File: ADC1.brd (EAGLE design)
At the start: 100 x 100 mm, 69 parts, among them IC1 STM32F303K8T6, IC2 TC7WZ07FK, IC3 ESP32-WROVER, J1 SJ-1608, J2 SJ-1608, J3 SJ-1608, J4 SJ-1608, J5 SJ-2012, J6 SJ-1608, J7 SJ-2012, J8 SJ-1608, X1 12MHz

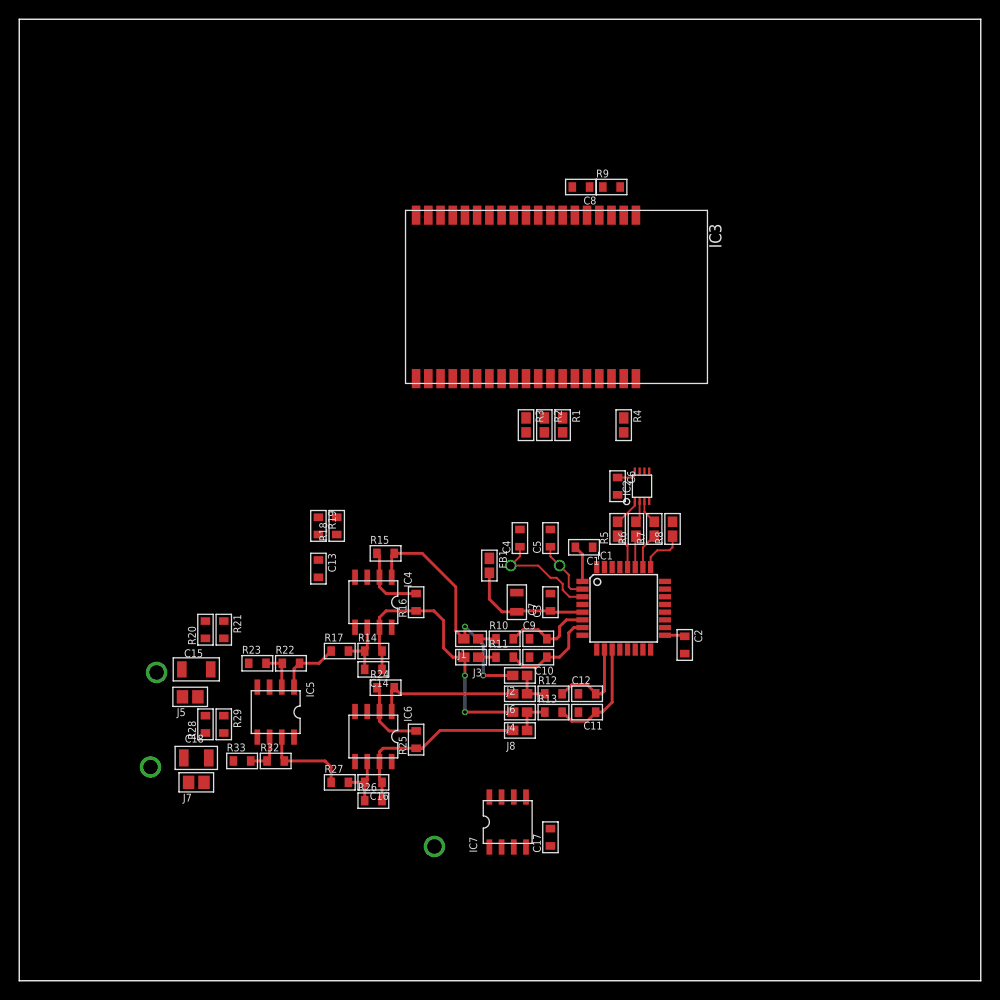
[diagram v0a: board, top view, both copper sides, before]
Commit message: ほぼ完成
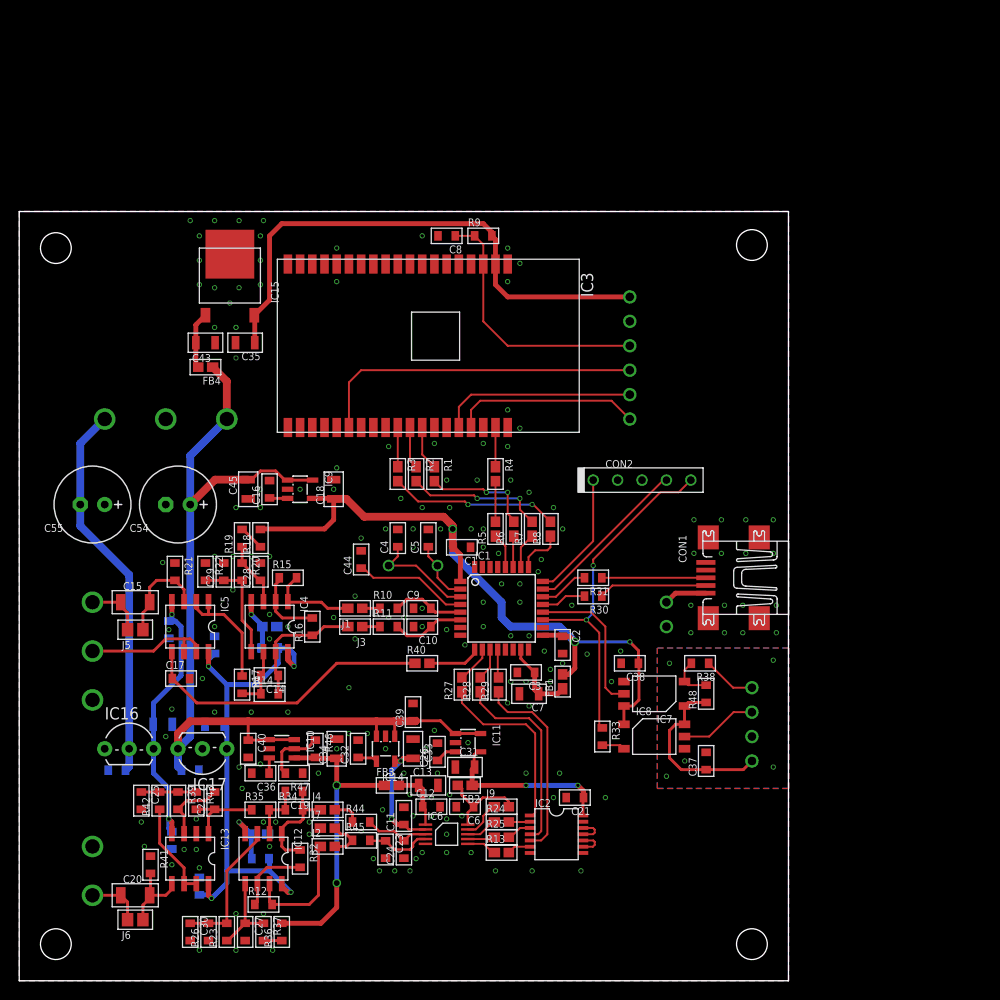
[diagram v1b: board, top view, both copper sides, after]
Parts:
- added C19, C25: 470p, my_rcl:1608
- added C20: 10u, my_rcl:3225
- added C21, C26, C27, C28, C29, C30, C32, C36, C37, C38, C39, C40, C41, C42, C44, C48, C49, C50, C51, C52, C53: 0.1u, my_rcl:1608
- added C22: 27p, my_rcl:1608
- added C23, C24: 1n, my_rcl:1608
- added C31, C33, C34, C35, C43, C45, C46, C47: 10u, my_rcl:2012
- added C54, C55: 100u, my_rcl:E2,5-8
- added CON1: USB-A, my_connector:UX60A-MB-5ST
- added CON2: SWD_CON, my_connector:SWD_CON
- added DR1, DR2, DR3, DR4: HOLE-3.2, my_connector:HOLE_3.2
- added FB2, FB3, FB4: FB, my_rcl:1608-J
- added IC10: NJM11100, my_ic:SOT23-6
- added IC11, IC9: 3.3V, my_ic:SOT23-5
- added IC12: LME49721, my_ic:SOP8
- added IC13: NJM4580, my_ic:SOP8
- added IC14: NJM12888F18, my_ic:SOT23-5
- added IC15: NJM2845-3.3, my_ic:P-HSIP3_2.30A
- added IC16: -5V, my_ic:TO-92
- added IC17: +5V, my_ic:TO-92
- added IC8: OCT_BUFFER-SO6, my_ic:SO6
- added J10, J9: SJ-1608, my_rcl:1608-J
- added R30, R31, R44, R45: 22, my_rcl:1608
- added R34, R35, R36, R37, R38, R39, R42, R43, R48: 1k, my_rcl:1608
- added R40: 0, my_rcl:1608-J
- added R41: 10k, my_rcl:1608
- added R46: 6.8k, my_rcl:1608
- added R47: 2.4k, my_rcl:1608
- added TP10: ESP_EN, my_connector:TESTPIN
- added TP11: ESP_BOOT, my_connector:TESTPIN
- added TP12: ESP_TX, my_connector:TESTPIN
- added TP13, TP20: GND, my_connector:TESTPIN
- added TP14: ESP_RX, my_connector:TESTPIN
- added TP15, TP16, TP18: GND, my_connector:TESTPIN-BIG
- added TP17: V+, my_connector:TESTPIN-BIG
- added TP19: V-, my_connector:TESTPIN-BIG
- added TP4: VBUS, my_connector:TESTPIN
- added TP5: UART_3V3, my_connector:TESTPIN
- added TP6: UART_RX, my_connector:TESTPIN
- added TP7: UART_GND, my_connector:TESTPIN
- added TP8: UART_TX, my_connector:TESTPIN
- added TP9: +3V3D, my_connector:TESTPIN
- C11: value 1n -> 0.1u
- C12: value 1n -> 3300p
- C13: value 0.1u -> 1u; device my_rcl:1608 -> my_rcl:2012
- C14: value (none) -> 27p
- C16: value (none) -> 0.1u
- C17: value (none) -> 470p
- C18: device my_rcl:3216 -> my_rcl:2012
- C7: value 1u -> 10u
- IC1: value STM32F303K8T6 -> STM32G431KB
- IC2: value TC7WZ07FK -> 7404; device my_ic:SOT765 -> my_ic:TSSOP14
- IC4: value (none) -> LME49721
- IC5: value (none) -> NJM4580
- IC6: value (none) -> MCP331X1; device my_ic:SOP8 -> my_ic:MSOP10
- IC7: value (none) -> OCT_BUFFER-SO6; device my_ic:SOP8 -> my_ic:SO6
- J5: value SJ-2012 -> IN3_DC
- J6: value SJ-1608 -> IN1_DC; device my_rcl:1608-J -> my_rcl:2012-J
- J7: value SJ-2012 -> SJ-1608; device my_rcl:2012-J -> my_rcl:1608-J
- R12: value 10 -> 1k
- R13: value 10 -> 37; device my_rcl:1608 -> my_rcl:1608-J
- R20: value 10k -> 1k
- R24, R25, R27: value 1k -> 37; device my_rcl:1608 -> my_rcl:1608-J
- R28, R29: value 10k -> 37; device my_rcl:1608 -> my_rcl:1608-J
- TP1: value AIN1 -> AIN3
- TP2: value AIN2 -> AIN1
- moved J6 46.4 mm to (12.1, 6.35)
- moved C17 41.8 mm to (16.8, 31.4), turned to 0 degrees
- moved TP3 41.0 mm to (7.62, 34.3)
- moved R33 37.6 mm to (60.6, 25.4), turned to 270 degrees
- moved R12 37.3 mm to (25.4, 7.94)
- moved IC2 37.3 mm to (55.9, 15.2), turned to 270 degrees
- moved C6 36.9 mm to (46.4, 18.1), turned to 180 degrees
- moved C16 32.3 mm to (26.0, 51.1), turned to 90 degrees
- moved C18 31.4 mm to (32.7, 51.1), turned to 90 degrees
- moved J8 29.1 mm to (25.1, 15.2), flipped to the bottom
- moved R28 28.9 mm to (47.9, 30.8)
- moved R29 28.9 mm to (49.8, 30.8), turned to 90 degrees
- moved R23 28.1 mm to (21.6, 5.08), turned to 90 degrees
- moved J2 26.8 mm to (32.1, 14.0)
- moved C13 25.3 mm to (42.5, 20.3), turned to 0 degrees
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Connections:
- removed net ADC2+: J2.2, J6.2, R12.1
- removed net ADC2-: J4.2, J8.2, R13.1
- removed net VCOM1: C13.1, IC4.3, IC4.5, IC6.3, IC6.5, R18.1, R19.2
- new net +1V8: C11.1, C33.1, IC14.5, IC6.2
- new net +5V: C41.1, C42.1, C46.1, C48.1, C50.1, IC12.8, IC13.8, IC17.1, IC4.8, IC5.8
- new net -5V: C47.2, C49.2, C51.2, IC13.4, IC16.3, IC5.4
- new net ADC3+: J1.2, R10.1
- new net ADC3-: J3.2, R11.1
- new net ADC_CNVST: IC2.5, R29.1
- new net ADC_SCK: IC2.1, R27.1
- new net ADC_SDO: IC2.4, R28.1
- new net ESP_BOOT: IC3.25, TP11.1
- new net N$32: CON1.2, R30.1
- new net N$33: CON1.3, R31.1
- new net N$35: IC7.3, R38.2, R48.2
- new net N$38: R36.1, R37.2
- new net N$39: C29.1, IC4.5, R20.2, R22.2
- new net N$40: R18.1, R19.2
- new net N$41: C27.1, IC12.5, R23.1, R37.1
- new net N$42: IC12.6, R12.1, R32.2
- new net N$43: C19.2, IC12.2, R34.1, R35.2
- new net N$44: C30.1, IC12.3, R23.2, R26.2
- new net N$45: IC13.6, IC13.7, R42.1
- new net N$46: IC12.7, J2.1, R12.2
- new net N$47: C19.1, IC12.1, J4.1, R32.1, R34.2
- new net N$48: C20.1, J6.1, TP2.1
- new net N$49: C20.2, IC13.5, J6.2, R41.2
- new net N$50: IC1.12, R29.2
- new net N$51: C16.1, IC9.3
- new net N$52: C24.2, IC6.3, R44.2
- new net N$53: C23.1, IC6.4, R45.2
- new net N$54: IC1.9, R40.2
- new net N$55: C22.2, IC13.3, R39.2
- new net N$56: C26.1, IC11.3
- new net N$57: C22.1, IC13.1, R35.1, R43.2
- new net N$58: IC2.11, IC2.12
- new net N$59: C32.1, IC14.4
- new net N$60: IC2.10, IC2.9
- new net N$61: C36.1, IC10.3
- new net N$62: IC10.5, R46.1, R47.2
- new net N$63: C42.2, IC12.4, J8.2
- new net N$64: C41.2, IC4.4, J10.2
- new net N$65: C43.1, FB4.2, IC15.1
- new net N$66: C44.1, IC1.4
- new net UART_3V3: C37.1, IC7.1, IC8.6, R48.1, TP5.1
- new net UART_GND: C37.2, IC8.4, TP7.1
- new net UART_RX: R38.1, TP6.1
- new net UART_TX: IC8.5, TP8.1
- new net USB_DM: IC1.21, R30.2
- new net USB_DP: IC1.22, R31.2
- new net VBUS: CON1.1, TP4.1
- new net VDDA: C3.1, C7.1, FB1.1, IC1.15
- new net VREF: C34.1, FB3.1, IC10.4, R36.2, R46.2
- net +3V3: now also C18.1, C38.1, FB1.2, IC7.6, IC8.1, IC9.4; no longer C6.1, FB1.1, IC2.8, R20.2, R28.2
- net +3V3A: now also C21.1, C31.1, FB2.1, IC11.4, IC2.14; no longer C3.1, C7.1, FB1.2, IC1.5
- net +3V3D: now also C35.1, IC15.3, TP9.1
- net ADC1+: now also J4.2, R44.1; no longer J1.2, R10.1
- net ADC1-: now also J2.2, J7.2, R45.1; no longer J3.2, R11.1
- net DAC1: now also IC5.5, R40.1; no longer IC1.12, IC7.3
- net ESP_EN: now also TP10.1
- net ESP_RX: now also TP14.1
- net ESP_TX: now also TP12.1
- net GND: now also C12.2, C16.2, C18.2, C21.2, C23.2, C24.1, C25.2, C26.2, C27.2, C28.2, C29.2, C30.2, C31.2, C32.2, C33.2, C34.2, C35.2, C36.2, C38.2, C39.2, C40.2, C43.2, C44.2, C45.2, C46.2, C47.1, C48.2, C49.1, C50.2, C51.1, C52.2, C53.1, C54.-, C55.+, CON1.5, CON1.M1, CON1.M2, CON1.M3, CON1.M4, CON2.3, IC1.14, IC1.31, IC10.2, IC11.2, IC13.2, IC14.2, IC15.2, IC16.1, IC17.2, IC2.7, IC2.8, IC6.5, IC7.4, IC9.2, J10.1, J7.1, J8.1, R22.1, R26.1, R41.1, R47.1, TP13.1, TP15.1, TP16.1, TP18.1, TP20.1; no longer C12.1, IC2.4, R19.1, R23.1, R29.1, R33.1
- net N$14: now also C28.1, IC4.3, R19.1, R20.1; no longer IC2.1, R5.2
- net N$15: now also C6.1, FB2.2, IC6.10, J9.2; no longer IC2.2, R6.2
- net N$16: now also C12.1, C13.1, FB3.2, IC6.1; no longer IC2.3, R7.2
- net N$19: now also IC2.6, R13.2; no longer C12.2, IC1.10, R12.2
- net N$2: now also IC1.5; no longer IC1.6
- net N$20: now also IC2.3, R25.2; no longer C11.1, IC1.11, R13.2
- net N$22: no longer R20.1
- net N$23: now also IC5.1, R17.1; no longer R22.1, R23.2
- net N$24: now also IC5.6, IC5.7; no longer IC7.1, IC7.2
- net N$25: now also IC6.7, R25.1; no longer C18.1, J7.1, TP2.1
- net N$26: no longer J2.1
- net N$27: no longer J4.1
- net N$28: now also IC6.8; no longer IC6.2, R25.2
- net N$29: now also IC6.6, R13.1; no longer C18.2, IC5.5, J7.2, R28.1, R29.2
- net N$30: now also IC6.9, J9.1; no longer C16.2, IC6.6, R26.1, R27.2
- net N$31: now also IC2.2, R24.2; no longer IC5.7, R27.1, R32.2
- net N$34: now also IC8.3; no longer IC5.6, R32.1
- net N$36: now also IC1.10, R27.2; no longer IC6.1, J6.1, R24.2
- net N$37: now also IC1.11, R28.2; no longer C16.1, IC6.7, J8.1, R25.1, R26.2
- net N$4: now also C25.1, R39.1, R42.2, R43.1; no longer IC5.1, R17.1, R22.2
- net N$5: now also IC1.6; no longer IC1.7
- net SPI_MISO: now also R6.2; no longer IC2.6
- net SPI_MOSI: now also R5.2; no longer IC2.7
- net SPI_SCK: now also R7.2; no longer IC2.5
- net STM_RX: now also IC1.20, IC7.5; no longer IC1.19
- net STM_TX: now also CON2.5, IC1.19, R33.1; no longer IC1.20
- net SWCLK: now also CON2.1
- net SWDIO: now also CON2.4
- net V+: now also C39.1, C40.1, C45.1, C52.1, C54.+, FB4.1, IC10.1, IC10.6, IC11.1, IC11.5, IC14.1, IC14.3, IC17.3, IC9.1, IC9.5, TP17.1; no longer IC4.8, IC5.8, IC6.8, IC7.8
- net V-: now also C53.2, C55.-, IC16.2, TP19.1; no longer IC4.4, IC5.4, IC6.4, IC7.4
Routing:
- net V+: track 0.00 -> 103.7 mm
- net +3V3: track 8.25 -> 76.3 mm, vias 0 -> 3
- net +3V3D: track 0.00 -> 55.9 mm
- net +5V: track 0.00 -> 55.2 mm, vias 0 -> 4
- net V-: track 0.00 -> 39.8 mm
- net STM_TX: track 0.00 -> 36.6 mm, vias 0 -> 2
- net ESP_BOOT: track 0.00 -> 34.4 mm
- net VREF: track 0.00 -> 31.3 mm, vias 0 -> 2
- net DAC1: track 0.00 -> 30.8 mm
- net -5V: track 0.00 -> 28.8 mm, vias 0 -> 2
- net ESP_EN: track 0.00 -> 27.6 mm
- net ADC_CNVST: track 0.00 -> 20.5 mm
- net ADC_SDO: track 0.00 -> 20.5 mm
- net ESP_RX: track 0.00 -> 20.5 mm
- net ESP_TX: track 0.00 -> 19.5 mm
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- added copper zone on layer 1, net GND
- added copper zone on layer 15, net GND
- added copper zone on layer 16, net GND
- added copper zone on layer 2, net GND
- added copper zone on layer 15, net N$67
- added copper zone on layer 2, net N$68
- added copper zone on layer 1, net UART_GND
- added copper zone on layer 16, net UART_GND
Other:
- board size 100 x 100 mm -> 80 x 80 mm
